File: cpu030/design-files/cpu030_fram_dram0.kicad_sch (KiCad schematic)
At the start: 36 parts, among them J201 DRAM0SZ, J202 DRAM0 JTAG, U201 ATF1508AS-TQFP100, U202 CY7C1061GE, U203 CY7C1061GE, U204 SIMM72-0A, U205 SIMM72-0B, U206 MC74ACT05DG

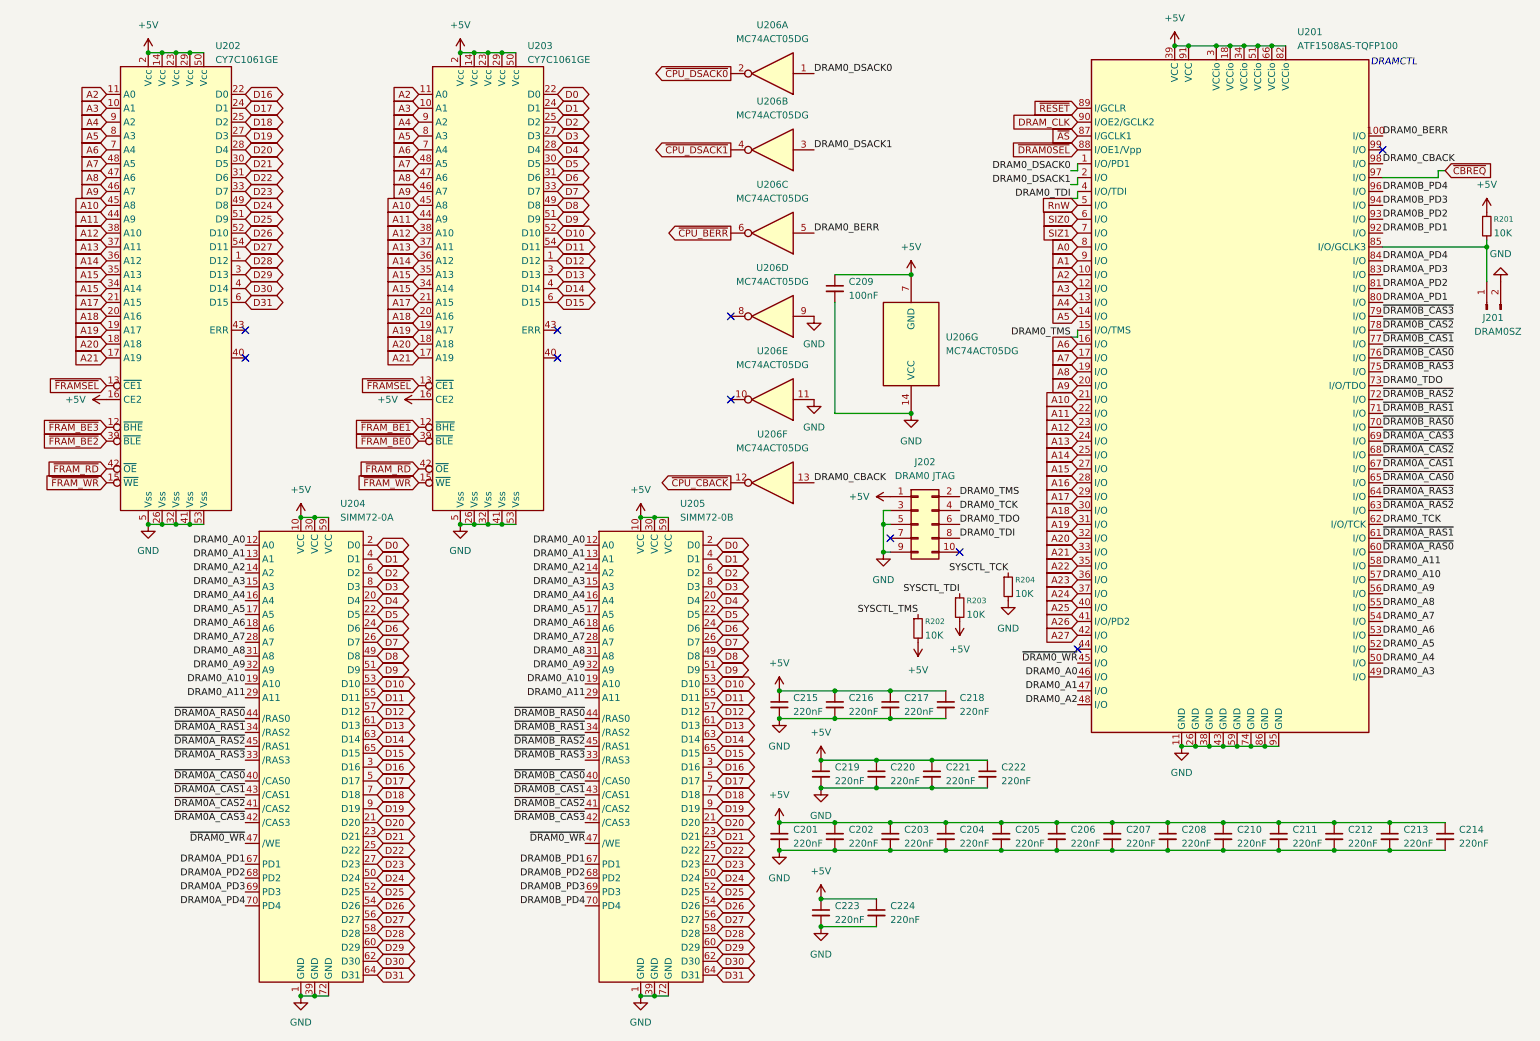
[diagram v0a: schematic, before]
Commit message: Group components with their caps.
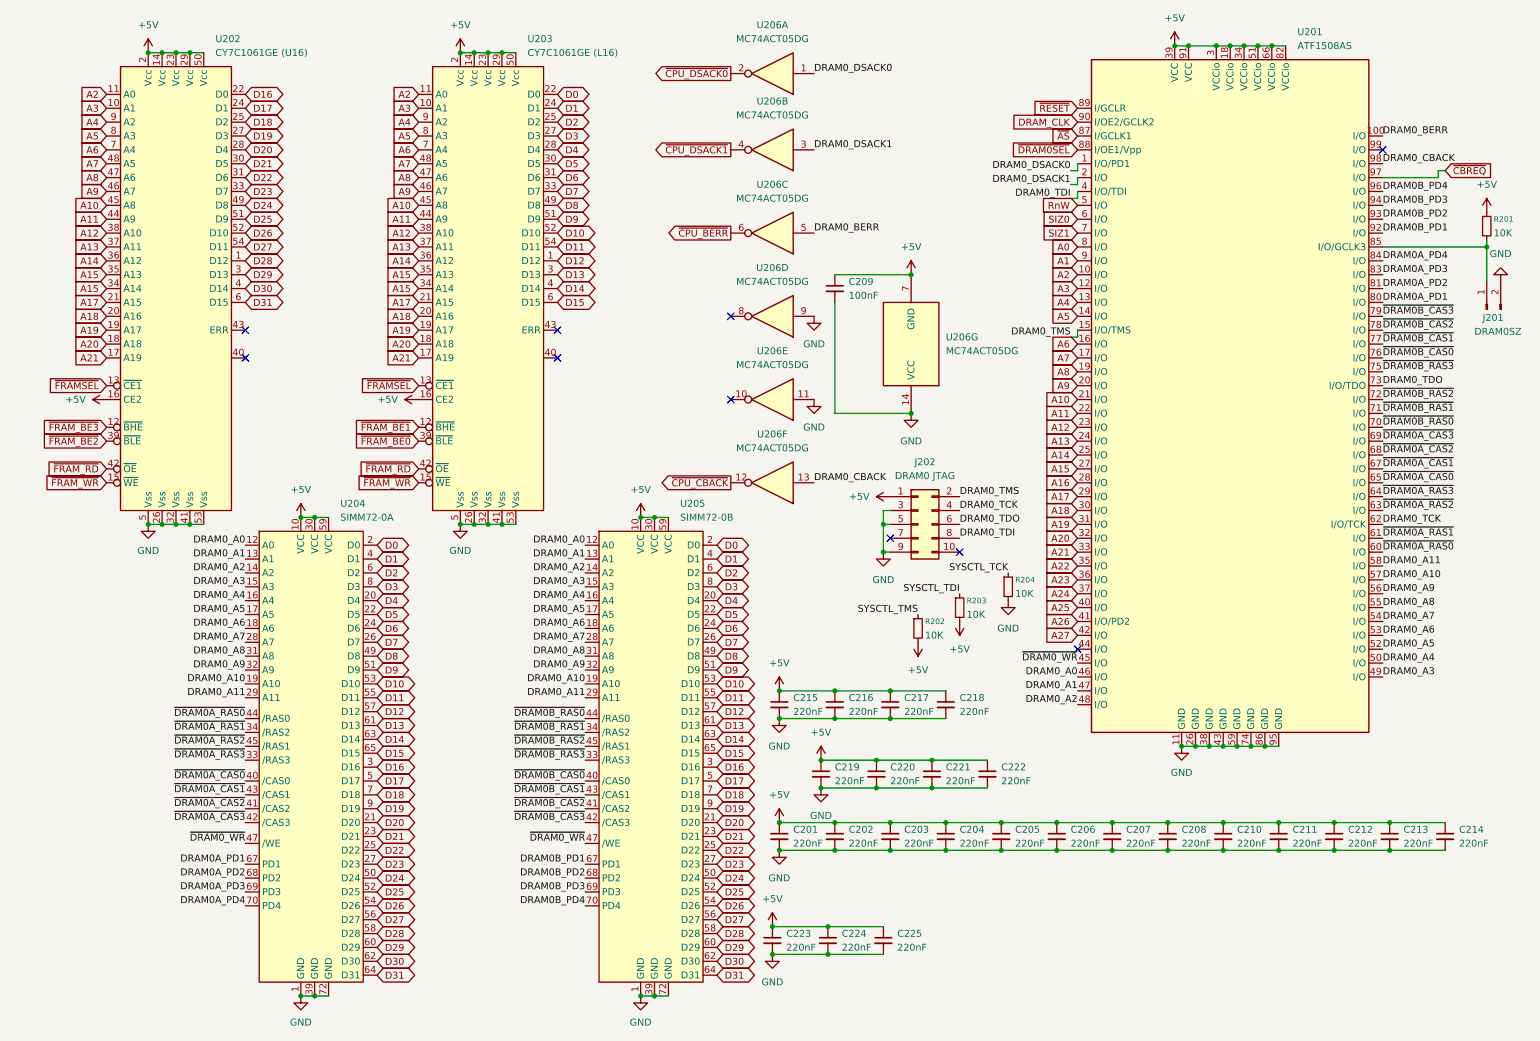
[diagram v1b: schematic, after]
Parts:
- added C225: 220nF, Capacitor_SMD:C_0805_2012Metric, symbol Device:C_Small
- U201: value ATF1508AS-TQFP100 -> ATF1508AS
- U202: value CY7C1061GE -> CY7C1061GE (U16)
- U203: value CY7C1061GE -> CY7C1061GE (L16)
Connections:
- net +5V: now also C225.1
- net GND: now also C225.2
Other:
- note removed: "DRAMCTL"
- moved on the sheet: C223, C224
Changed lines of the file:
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@@
 	(generator_version "9.0")
 	(paper "A4")
-	(text "DRAMCTL"
-		(exclude_from_sim no)
-		(at 261.112 20.828 0)
-		(effects
-			(font
-				(size 1.27 1.27)
-				(italic yes)
-			)
-		)
-	)
 	(junction
 		(at 158.75 135.89)
@@
 	)
 	(junction
+		(at 157.48 179.07)
+		(diameter 0)
+		(color 0 0 0 0)
+	)
+	(junction
 		(at 158.75 160.02)
 		(diameter 0)
@@
 	)
 	(junction
-		(at 156.21 173.99)
+		(at 147.32 179.07)
 		(diameter 0)
 		(color 0 0 0 0)
@@
 	)
 	(junction
-		(at 156.21 179.07)
+		(at 147.32 184.15)
 		(diameter 0)
 		(color 0 0 0 0)
@@
 	)
 	(junction
+		(at 157.48 184.15)
+		(diameter 0)
+		(color 0 0 0 0)
+	)
+	(junction
 		(at 97.79 105.41)
 		(diameter 0)
@@
 	(wire
 		(pts
-			(xy 156.21 179.07) (xy 166.37 179.07)
+			(xy 147.32 184.15) (xy 157.48 184.15)
 		)
 		(stroke
@@
 	(wire
 		(pts
-			(xy 156.21 173.99) (xy 166.37 173.99)
+			(xy 157.48 179.07) (xy 167.64 179.07)
+		)
+		(stroke
+			(width 0)
+			(type default)
+		)
+	)
+	(wire
+		(pts
+			(xy 147.32 179.07) (xy 157.48 179.07)
 		)
 		(stroke
@@
 	(wire
 		(pts
+			(xy 157.48 184.15) (xy 167.64 184.15)
+		)
+		(stroke
+			(width 0)
+			(type default)
+		)
+	)
+	(wire
+		(pts
 			(xy 168.91 102.87) (xy 167.64 102.87)
 		)
@@
 	(symbol
 		(lib_id "Device:C_Small")
-		(at 156.21 176.53 0)
+		(at 147.32 181.61 0)
 		(unit 1)
 		(exclude_from_sim no)
@@
 		(fields_autoplaced yes)
 		(property "Reference" "C223"
-			(at 158.75 175.2662 0)
+			(at 149.86 180.3462 0)
 			(effects
 				(font
@@
 		)
 		(property "Value" "220nF"
-			(at 158.75 177.8062 0)
+			(at 149.86 182.8862 0)
 			(effects
 				(font
@@
 		)
 		(property "Footprint" "Capacitor_SMD:C_0805_2012Metric"
-			(at 156.21 176.53 0)
+			(at 147.32 181.61 0)
 			(effects
 				(font
@@
 		)
 		(property "Datasheet" "~"
-			(at 156.21 176.53 0)
+			(at 147.32 181.61 0)
 			(effects
 				(font
@@
 		)
 		(property "Description" "Unpolarized capacitor, small symbol"
-			(at 156.21 176.53 0)
+			(at 147.32 181.61 0)
 			(effects
 				(font
@@
 	(symbol
 		(lib_id "power:+5V")
-		(at 156.21 173.99 0)
+		(at 147.32 179.07 0)
 		(unit 1)
 		(exclude_from_sim no)
@@
 		(dnp no)
 		(property "Reference" "#PWR0230"
-			(at 156.21 177.8 0)
+			(at 147.32 182.88 0)
 			(effects
 				(font
@@
 		)
 		(property "Value" "+5V"
-			(at 156.21 168.91 0)
+			(at 147.32 173.99 0)
 			(effects
 				(font
@@
 		)
 		(property "Footprint" ""
-			(at 156.21 173.99 0)
+			(at 147.32 179.07 0)
 			(effects
 				(font
@@
 		)
 		(property "Datasheet" ""
-			(at 156.21 173.99 0)
+			(at 147.32 179.07 0)
 			(effects
 				(font
@@
 		)
 		(property "Description" "Power symbol creates a global label with name \"+5V\""
-			(at 156.21 173.99 0)
+			(at 147.32 179.07 0)
 			(effects
 				(font
@@
 	(symbol
 		(lib_id "power:GND")
-		(at 156.21 179.07 0)
+		(at 147.32 184.15 0)
 		(unit 1)
 		(exclude_from_sim no)
@@
 		(fields_autoplaced yes)
 		(property "Reference" "#PWR0231"
-			(at 156.21 185.42 0)
+			(at 147.32 190.5 0)
 			(effects
 				(font
@@
 		)
 		(property "Value" "GND"
-			(at 156.21 184.15 0)
+			(at 147.32 189.23 0)
 			(effects
 				(font
@@
 		)
 		(property "Footprint" ""
-			(at 156.21 179.07 0)
+			(at 147.32 184.15 0)
 			(effects
 				(font
@@
 		)
 		(property "Datasheet" ""
-			(at 156.21 179.07 0)
+			(at 147.32 184.15 0)
 			(effects
 				(font
@@
 		)
 		(property "Description" "Power symbol creates a global label with name \"GND\" , ground"
-			(at 156.21 179.07 0)
+			(at 147.32 184.15 0)
 			(effects
 				(font
@@
 			)
 		)
-		(property "Value" "ATF1508AS-TQFP100"
+		(property "Value" "ATF1508AS"
 			(at 243.4433 17.78 0)
 			(effects
@@
 	)
 	(symbol
+		(lib_id "Device:C_Small")
+		(at 167.64 181.61 0)
+		(unit 1)
+		(exclude_from_sim no)
+		(in_bom yes)
+		(on_board yes)
+		(dnp no)
+		(fields_autoplaced yes)
+		(property "Reference" "C225"
+			(at 170.18 180.3462 0)
+			(effects
+				(font
+					(size 1.27 1.27)
+				)
+				(justify left)
+			)
+		)
+		(property "Value" "220nF"
+			(at 170.18 182.8862 0)
+			(effects
+				(font
+					(size 1.27 1.27)
+				)
+				(justify left)
+			)
+		)
+		(property "Footprint" "Capacitor_SMD:C_0805_2012Metric"
+			(at 167.64 181.61 0)
+			(effects
+				(font
+					(size 1.27 1.27)
+				)
+				(hide yes)
+			)
+		)
+		(property "Datasheet" "~"
+			(at 167.64 181.61 0)
+			(effects
+				(font
+					(size 1.27 1.27)
+				)
+				(hide yes)
+			)
+		)
+		(property "Description" "Unpolarized capacitor, small symbol"
+			(at 167.64 181.61 0)
+			(effects
+				(font
+					(size 1.27 1.27)
+				)
+				(hide yes)
+			)
+		)
+		(pin "1"
+		)
+		(pin "2"
+		)
+		(instances
+			(project "cpu030"
+				(path "/6696b89f-f6cc-4e49-bcfb-68bdb218d2a6/6473b99a-f5fc-46a4-ae73-90633955ad5d"
+					(reference "C225")
+					(unit 1)
+				)
+			)
+		)
+	)
+	(symbol
 		(lib_id "power:GND")
 		(at 190.5 119.38 0)
@@
 	(symbol
 		(lib_id "Device:C_Small")
-		(at 166.37 176.53 0)
+		(at 157.48 181.61 0)
 		(unit 1)
 		(exclude_from_sim no)
@@
 		(fields_autoplaced yes)
 		(property "Reference" "C224"
-			(at 168.91 175.2662 0)
+			(at 160.02 180.3462 0)
 			(effects
 				(font
@@
 		)
 		(property "Value" "220nF"
-			(at 168.91 177.8062 0)
+			(at 160.02 182.8862 0)
 			(effects
 				(font
@@
 		)
 		(property "Footprint" "Capacitor_SMD:C_0805_2012Metric"
-			(at 166.37 176.53 0)
+			(at 157.48 181.61 0)
 			(effects
 				(font
@@
 		)
 		(property "Datasheet" "~"
-			(at 166.37 176.53 0)
+			(at 157.48 181.61 0)
 			(effects
 				(font
@@
 		)
 		(property "Description" "Unpolarized capacitor, small symbol"
-			(at 166.37 176.53 0)
+			(at 157.48 181.61 0)
 			(effects
 				(font
@@
 		(fields_autoplaced yes)
 		(property "Reference" "U203"
-			(at 102.4733 17.78 0)
+			(at 102.4733 16.51 0)
 			(effects
 				(font
@@
 			)
 		)
-		(property "Value" "CY7C1061GE"
-			(at 102.4733 20.32 0)
+		(property "Value" "CY7C1061GE (L16)"
+			(at 102.4733 19.05 0)
 			(effects
 				(font
@@
 		(fields_autoplaced yes)
 		(property "Reference" "U202"
-			(at 45.3233 17.78 0)
+			(at 45.3233 16.51 0)
 			(effects
 				(font
@@
 			)
 		)
-		(property "Value" "CY7C1061GE"
-			(at 45.3233 20.32 0)
+		(property "Value" "CY7C1061GE (U16)"
+			(at 45.3233 19.05 0)
 			(effects
 				(font
